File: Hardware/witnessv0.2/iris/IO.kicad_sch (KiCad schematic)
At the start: 18 parts, among them J2 Conn_01x02, J3 USB_B_Micro, J5 Conn_01x04, J6 Conn_01x04, J7 Conn_01x04, J8 Conn_01x04, U3 LTV-817S, U5 TCAN1044A-Q1, U9 USBLC6-2SC6

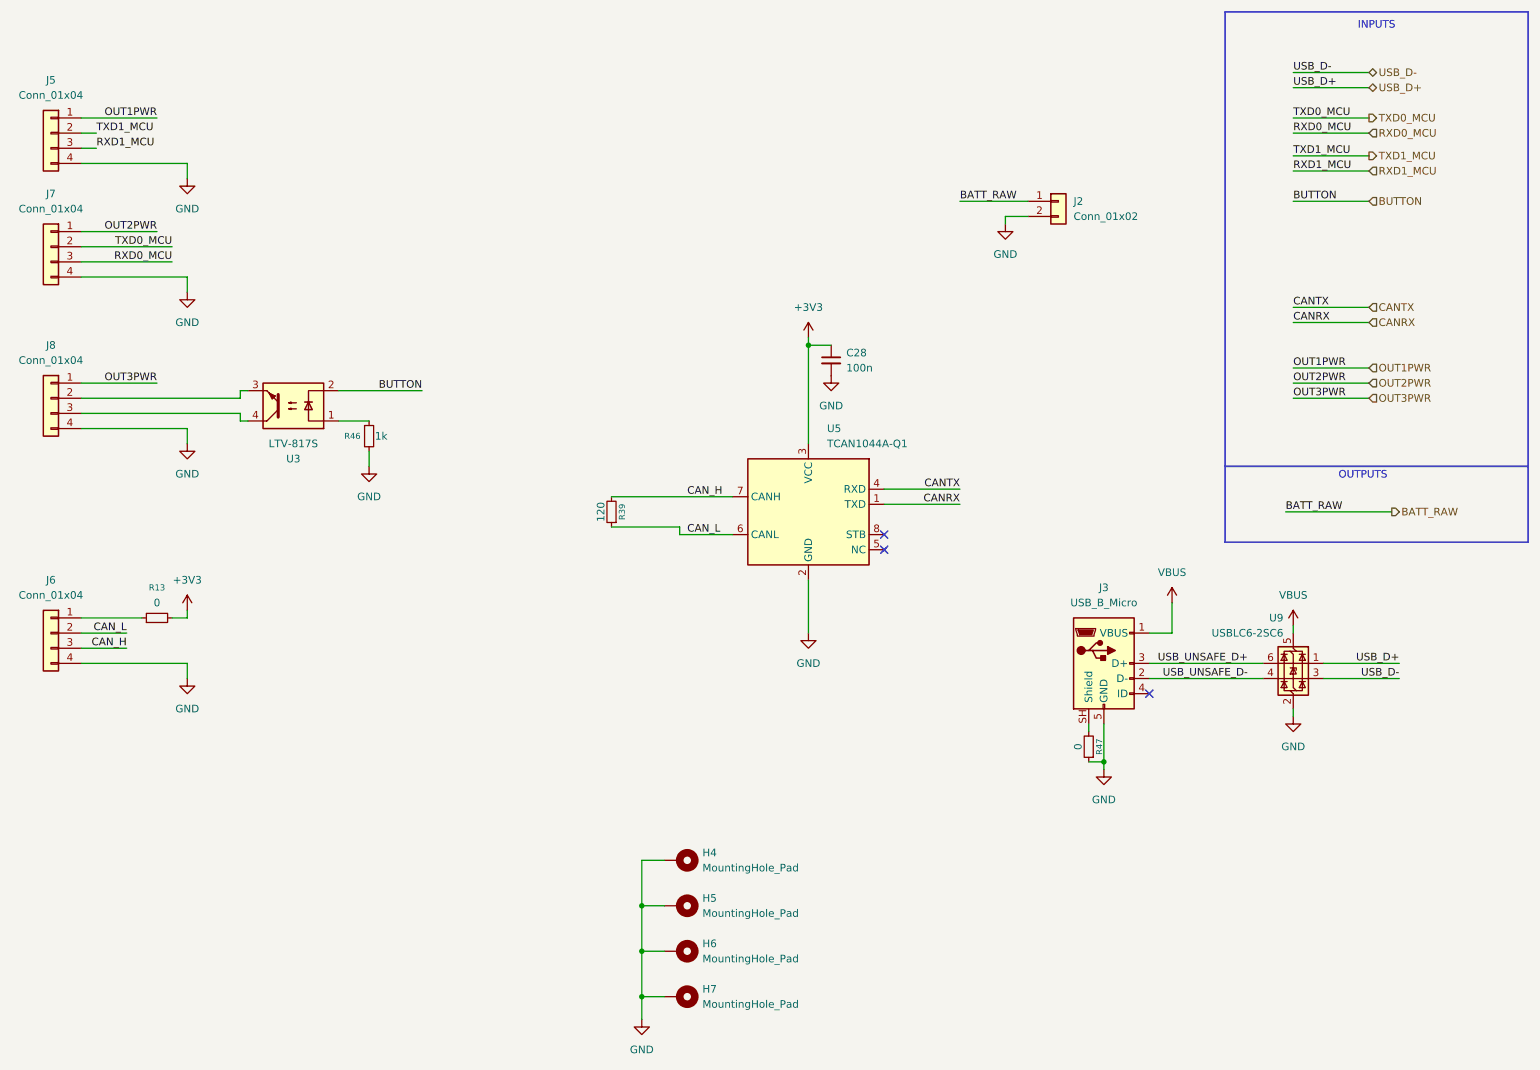
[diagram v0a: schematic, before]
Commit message: root feedback
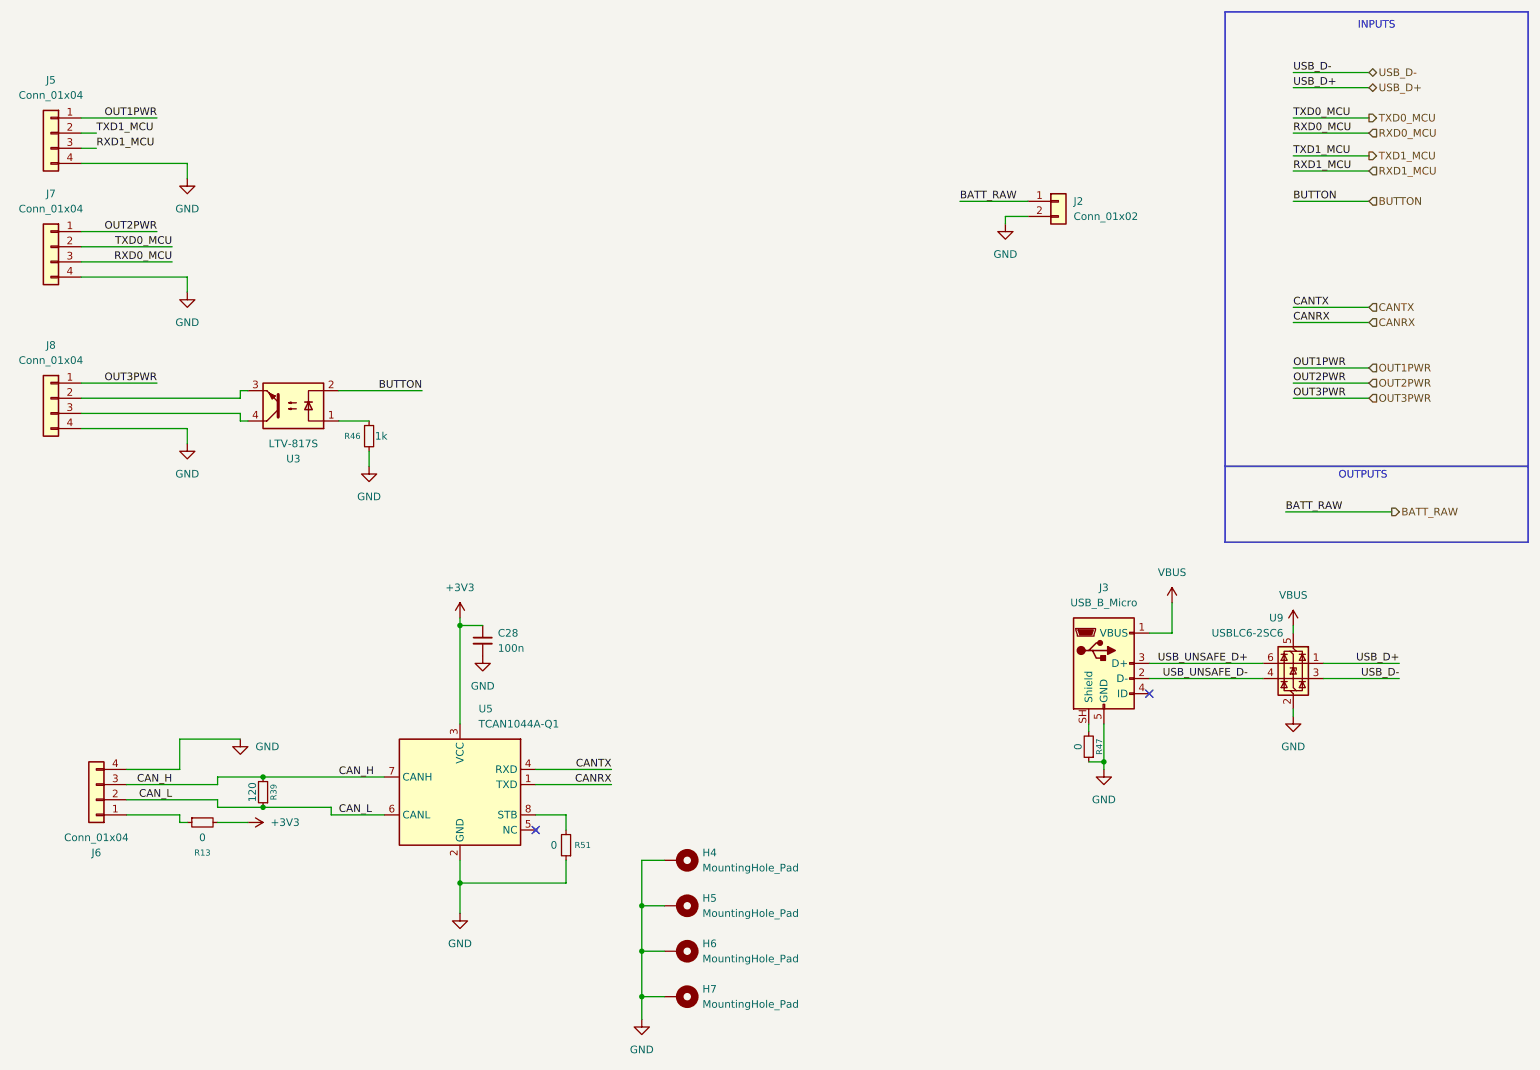
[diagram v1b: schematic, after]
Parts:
- added R51: 0, Resistor_SMD:R_0402_1005Metric, symbol Device:R_Small
- R13: LCSC_Part (none) -> C21189
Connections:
- net GND: now also R51.1
- net at U5.8 (STB): now also R51.2
- no-connect marks 3 -> 2
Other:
- moved on the sheet: C28, J6, R13, R39, U5
